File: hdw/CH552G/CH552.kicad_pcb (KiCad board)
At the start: 2 copper layers, 34.3 x 19.3 mm, 19 parts, among them J1 USB_A, J2 Conn_01x07, J3 Conn_01x07, SW1 RST, SW2 BOOT, U1 CH552G

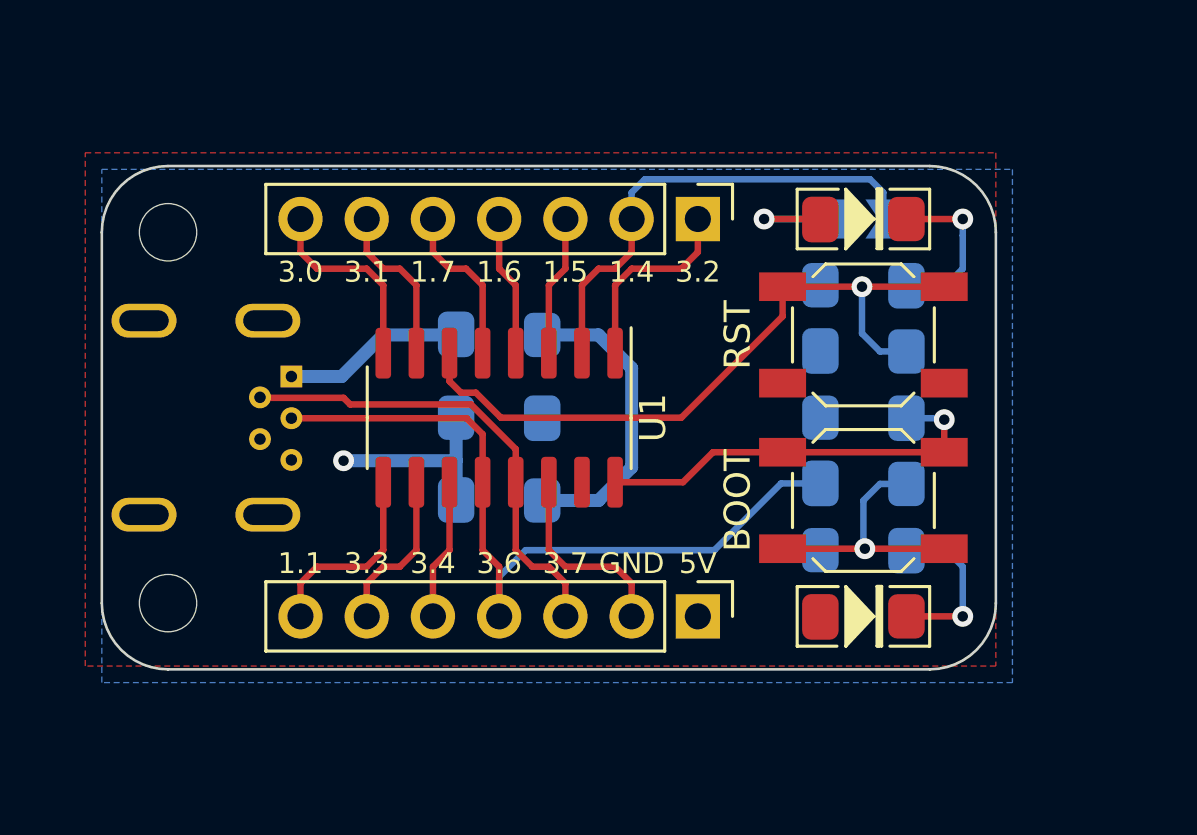
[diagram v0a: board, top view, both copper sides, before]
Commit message: feat - breakout CH552G v2.0
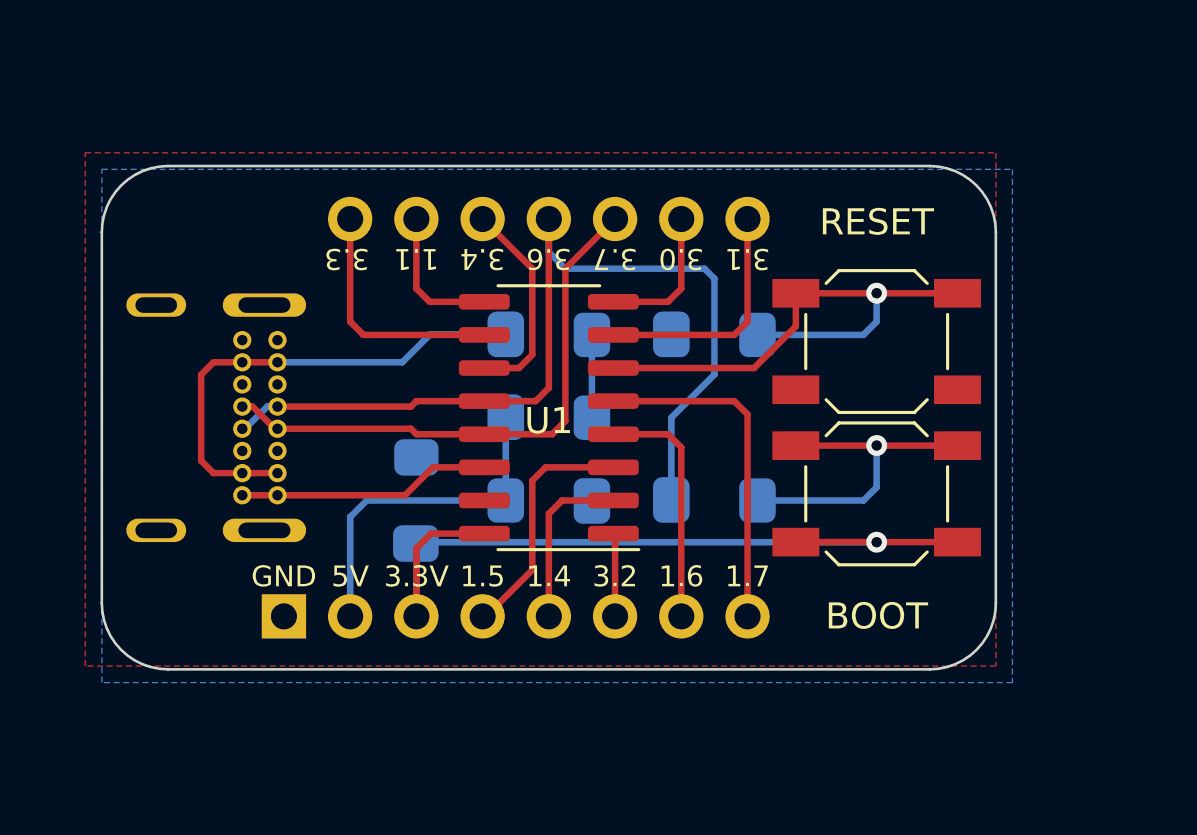
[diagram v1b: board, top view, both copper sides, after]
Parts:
- removed the D1 at (158.8, 109.2)
- removed D2: LED, Library:L1206
- removed H1, H2: MountingHole, MountingHole:MountingHole_2.2mm_M2
- removed J2: Conn_01x07, Connector_PinHeader_2.54mm:PinHeader_1x07_P2.54mm_Vertical
- removed JP1: SolderJumper_2_Open, Library:SolderJumper
- removed the R1 at (158.8, 111.8)
- removed R4: 1k, Library:R1206
- added P1: USB_C_Plug_USB2.0, Library:USB_C_MC_112D, F.Cu at (132.7, 116.8)
- J1: value USB_A -> Conn_01x08; footprint Library:USB_Micro-B -> Connector_PinHeader_2.54mm:PinHeader_1x08_P2.54mm_Vertical
- SW1: value RST -> RESET
- moved C1 17.4 mm to (141.6, 120.0), turned to -90 degrees
- moved J3 15.4 mm to (154.3, 109.2)
- moved J1 8.03 mm to (136.5, 124.5), turned to 90 degrees
- moved R2 5.75 mm to (153.0, 120.0)
- moved R1 5.75 mm to (153.0, 113.7)
- moved C2 3.70 mm to (146.7, 120.0)
- moved F1 3.70 mm to (146.7, 116.8)
- moved D1 1.91 mm to (146.7, 113.7)
- moved U1 1.91 mm to (146.7, 116.8), turned to 180 degrees
- moved SW2 0.57 mm to (159.3, 119.8), turned to 180 degrees
- moved SW1 0.57 mm to (159.3, 113.9)
- renumbered D3 to D1, R2 to R1, R3 to R2
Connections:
- J1 pad 1: VBUS -> GND
- J1 pad 2: P3.7 -> +5V
- J1 pad 3: P3.6 -> V33
- J1 pad 4: GND -> P1.5
- J1 pad 5: unconnected-(J1-Shield-Pad5) -> P1.4
- J1 pad 6: (no net) -> P3.2
- J3 pad 1: +5V -> P3.1
- J3 pad 2: GND -> P3.0
- J3 pad 6: P3.3 -> P1.1
- J3 pad 7: P1.1 -> P3.3
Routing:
- net V33: track 15.8 -> 32.2 mm
- net VBUS: track 6.99 -> 18.7 mm
- net P1.4: track 18.4 -> 6.62 mm
- net Net-(D1-K): track 11.7 -> 3.17 mm
- net P1.7: track 6.31 -> 13.1 mm
- net Net-(D1-K) (its old number): track 6.49 -> 0.00 mm, vias 1 -> 0
- net Net-(D2-K): track 6.49 -> 0.00 mm, vias 1 -> 0
- net RST: track 27.2 -> 21.0 mm
- net P3.6: track 30.2 -> 36.1 mm
- net +5V: track 7.47 -> 13.2 mm, vias 1 -> 0
- net Net-(D1-A): track 5.22 -> 0.00 mm, vias 1 -> 0
- net P3.2: track 7.58 -> 3.20 mm
- net P1.5: track 5.41 -> 9.39 mm
- net P1.6: track 5.41 -> 9.29 mm
- net P3.7: track 18.2 -> 21.6 mm
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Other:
- board text added: "3.3V"
- board text added: "V2 2024/01"
- board text removed: "V1.1 2023/04"

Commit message: wip
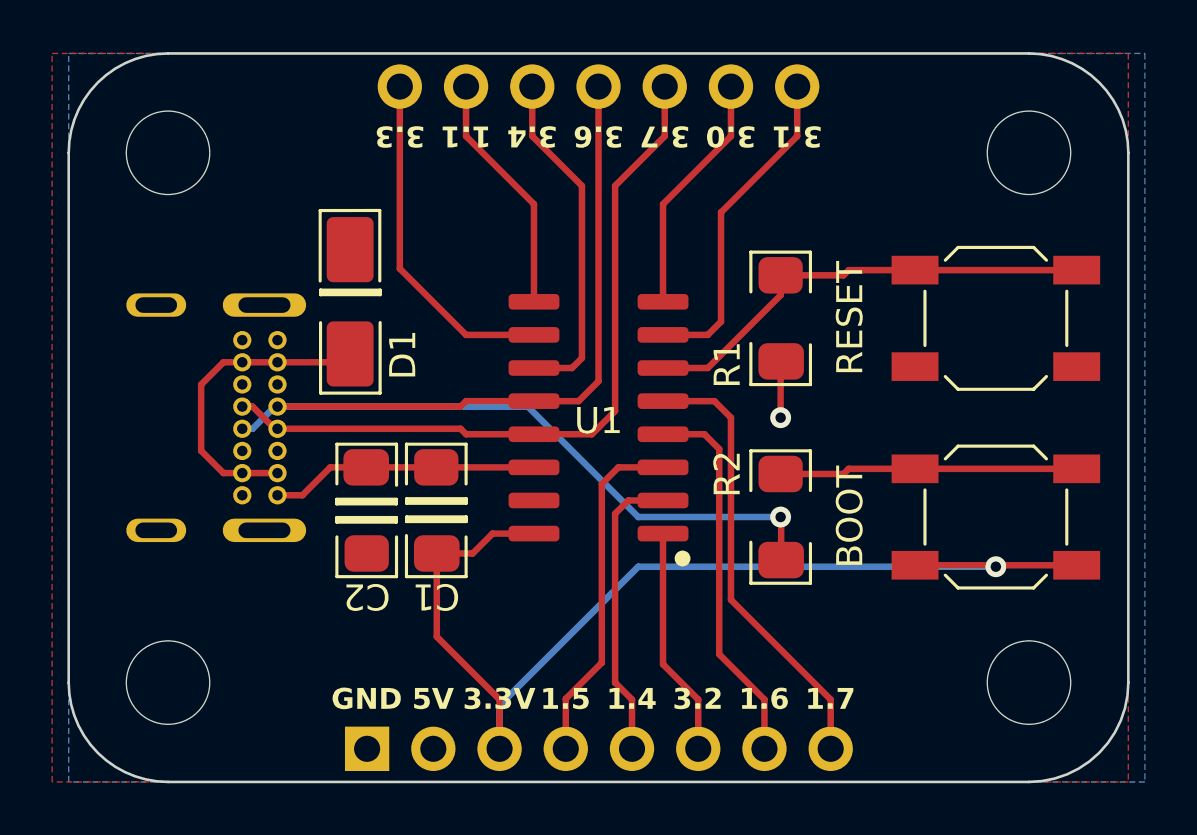
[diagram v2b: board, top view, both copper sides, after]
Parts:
- removed F1: Polyfuse, Library:F1206
- added H1: MountingHole, MountingHole:MountingHole_3.2mm_M3, F.Cu at (132.1, 106.7)
- added H2: MountingHole, MountingHole:MountingHole_3.2mm_M3, F.Cu at (165.1, 106.7)
- added H3: MountingHole, MountingHole:MountingHole_3.2mm_M3, F.Cu at (165.1, 127.0)
- added H4: MountingHole, MountingHole:MountingHole_3.2mm_M3, F.Cu at (132.1, 127.0)
- C1, C2, R1, R2: moved to F.Cu
- D1: footprint Library:D1206 -> Library:SMA_DO_214AC; moved to F.Cu
- P1: value USB_C_Plug_USB2.0 -> USB_C_Receptacle_USB2.0
- moved D1 7.73 mm to (139.1, 112.4), turned to 90 degrees
- moved C2 7.00 mm to (139.7, 120.4), turned to 90 degrees
- moved J1 6.00 mm to (139.7, 129.5)
- moved J3 5.43 mm to (156.2, 104.1)
- moved SW2 4.66 mm to (163.8, 120.7)
- moved SW1 4.66 mm to (163.8, 113.0)
- moved R1 2.62 mm to (155.6, 113.0), turned to -90 degrees
- moved R2 2.62 mm to (155.6, 120.7), turned to -90 degrees
- moved U1 1.91 mm to (148.6, 116.8)
- moved C1 0.85 mm to (142.4, 120.4)
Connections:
- D1 pad 1: Net-(D1-K) -> +5V
- P1 pad A8: (no net) -> unconnected-(P1-SBU1-PadA8)
- P1 pad B6: (no net) -> P3.6
- P1 pad B7: (no net) -> P3.7
- P1 pad B8: (no net) -> unconnected-(P1-SBU2-PadB8)
- P1 pad S1: unconnected-(P1-SHIELD-PadS1) -> GND
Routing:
- net +5V: track 13.2 -> 0.00 mm
- net P3.6: track 36.1 -> 48.4 mm, vias 0 -> 1
- net V33: track 32.2 -> 41.7 mm
- net P3.7: track 21.6 -> 28.3 mm
- net VBUS: track 18.7 -> 12.0 mm
- net P3.2: track 3.20 -> 8.81 mm
- net P1.6: track 9.29 -> 14.6 mm
- net P3.4: track 8.05 -> 13.2 mm
- net P1.4: track 6.62 -> 11.3 mm
- net P1.7: track 13.1 -> 17.2 mm
- net P1.5: track 9.39 -> 13.3 mm
- net P3.3: track 9.29 -> 13.2 mm
- net P1.1: track 5.48 -> 9.33 mm
- net P3.0: track 5.48 -> 9.33 mm
- net P3.1: track 9.29 -> 12.7 mm
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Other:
- board size 34.3 x 19.3 mm -> 40.6 x 27.9 mm
- board text added: "V3.1 2024-04"
- board text added: "nicola@strappazzon.me"
- board text removed: "V2 2024/01"
- board text removed: "nstrappazzonc"
